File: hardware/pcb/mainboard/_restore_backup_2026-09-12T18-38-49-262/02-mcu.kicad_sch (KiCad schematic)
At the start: 9 parts, among them SW2 RESET, SW3 BOOT, U1 ESP32-S3-WROOM-1-N16R8

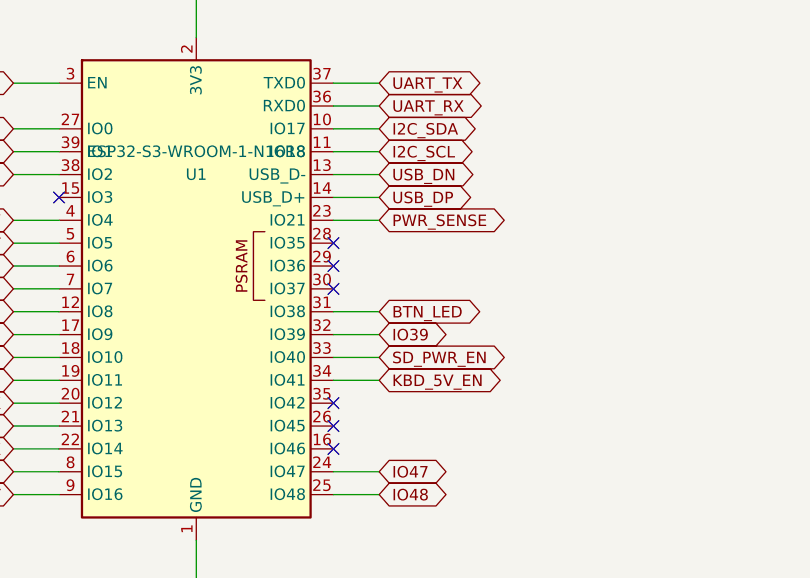
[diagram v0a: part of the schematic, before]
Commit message: Update mainboard
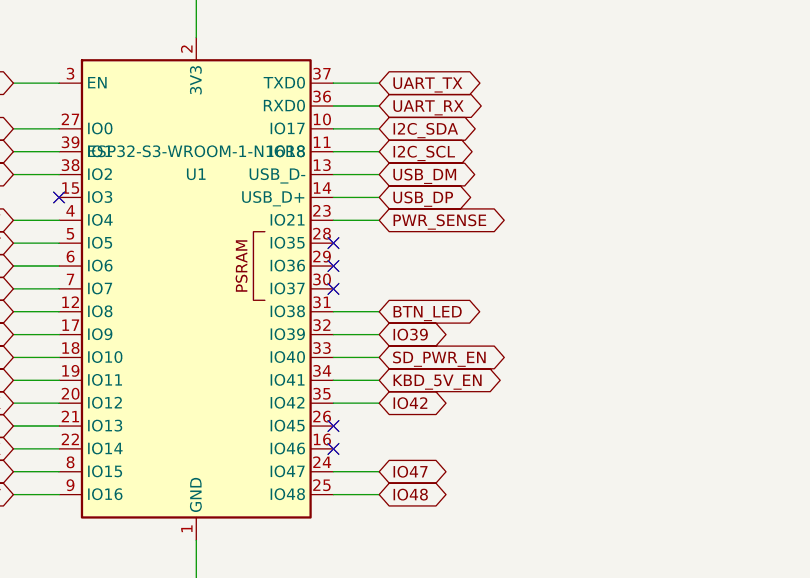
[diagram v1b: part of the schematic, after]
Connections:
- net IO42: now reaches U1.35 (IO42)
- net USB_DN renamed USB_DM
- no-connect marks 7 -> 6
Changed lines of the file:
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@@
+	(wire
+		(pts
+			(xy 322.58 97.79) (xy 327.66 97.79)
+		)
+		(stroke
+			(width 0)
+			(type default)
+		)
+	)
 	(wire
 		(pts
@@
 		)
 	)
+	(global_label "IO42"
+		(shape bidirectional)
+		(at 327.66 97.79 0)
+		(fields_autoplaced yes)
+		(effects
+			(font
+				(size 1.27 1.27)
+			)
+			(justify left)
+		)
+		(property "Intersheetrefs" "${INTERSHEET_REFS}"
+			(at 327.66 97.79 0)
+			(hide yes)
+			(show_name no)
+			(do_not_autoplace no)
+			(effects
+				(font
+					(size 1.27 1.27)
+				)
+			)
+		)
+	)
 	(global_label "IO48"
 		(shape bidirectional)
@@
 		)
 	)
-	(global_label "USB_DN"
+	(global_label "USB_DM"
 		(shape bidirectional)
 		(at 327.66 72.39 0)
@@
 		)
 	)
-	(no_connect
-		(at 322.58 97.79)
-	)
 )
